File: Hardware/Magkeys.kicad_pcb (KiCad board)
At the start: 2 copper layers, 338 x 114.6 mm, 203 parts, among them SW1 SW_Push, SW10 SW_Push, SW100 SW_Push, SW101 SW_Push, SW11 SW_Push, SW12 SW_Push, SW13 SW_Push, SW14 SW_Push, SW15 SW_Push, SW16 SW_Push, SW17 SW_Push, SW18 SW_Push, SW19 SW_Push, SW2 SW_Push, SW20 SW_Push, SW21 SW_Push, SW22 SW_Push, SW23 SW_Push, SW24 SW_Push, SW25 SW_Push, SW26 SW_Push, SW27 SW_Push, SW28 SW_Push, SW29 SW_Push, SW3 SW_Push, SW30 SW_Push, SW31 SW_Push, SW32 SW_Push, SW33 SW_Push, SW34 SW_Push, SW35 SW_Push, SW36 SW_Push, SW37 SW_Push, SW38 SW_Push, SW39 SW_Push, SW4 SW_Push, SW40 SW_Push, SW41 SW_Push, SW42 SW_Push, SW43 SW_Push, SW44 SW_Push, SW45 SW_Push, SW46 SW_Push, SW47 SW_Push, SW48 SW_Push, SW49 SW_Push, SW5 SW_Push, SW50 SW_Push, SW51 SW_Push, SW52 SW_Push, SW53 SW_Push, SW54 SW_Push, SW55 SW_Push, SW56 SW_Push, SW57 SW_Push, SW58 SW_Push, SW59 SW_Push, SW6 SW_Push, SW60 SW_Push, SW61 SW_Push, SW62 SW_Push, SW63 SW_Push, SW64 SW_Push, SW65 SW_Push, SW66 SW_Push, SW67 SW_Push, SW68 SW_Push, SW69 SW_Push, SW7 SW_Push, SW70 SW_Push, SW71 SW_Push, SW72 SW_Push, SW73 SW_Push, SW74 SW_Push, SW75 SW_Push, SW76 SW_Push, SW77 SW_Push, SW78 SW_Push, SW79 SW_Push, SW8 SW_Push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

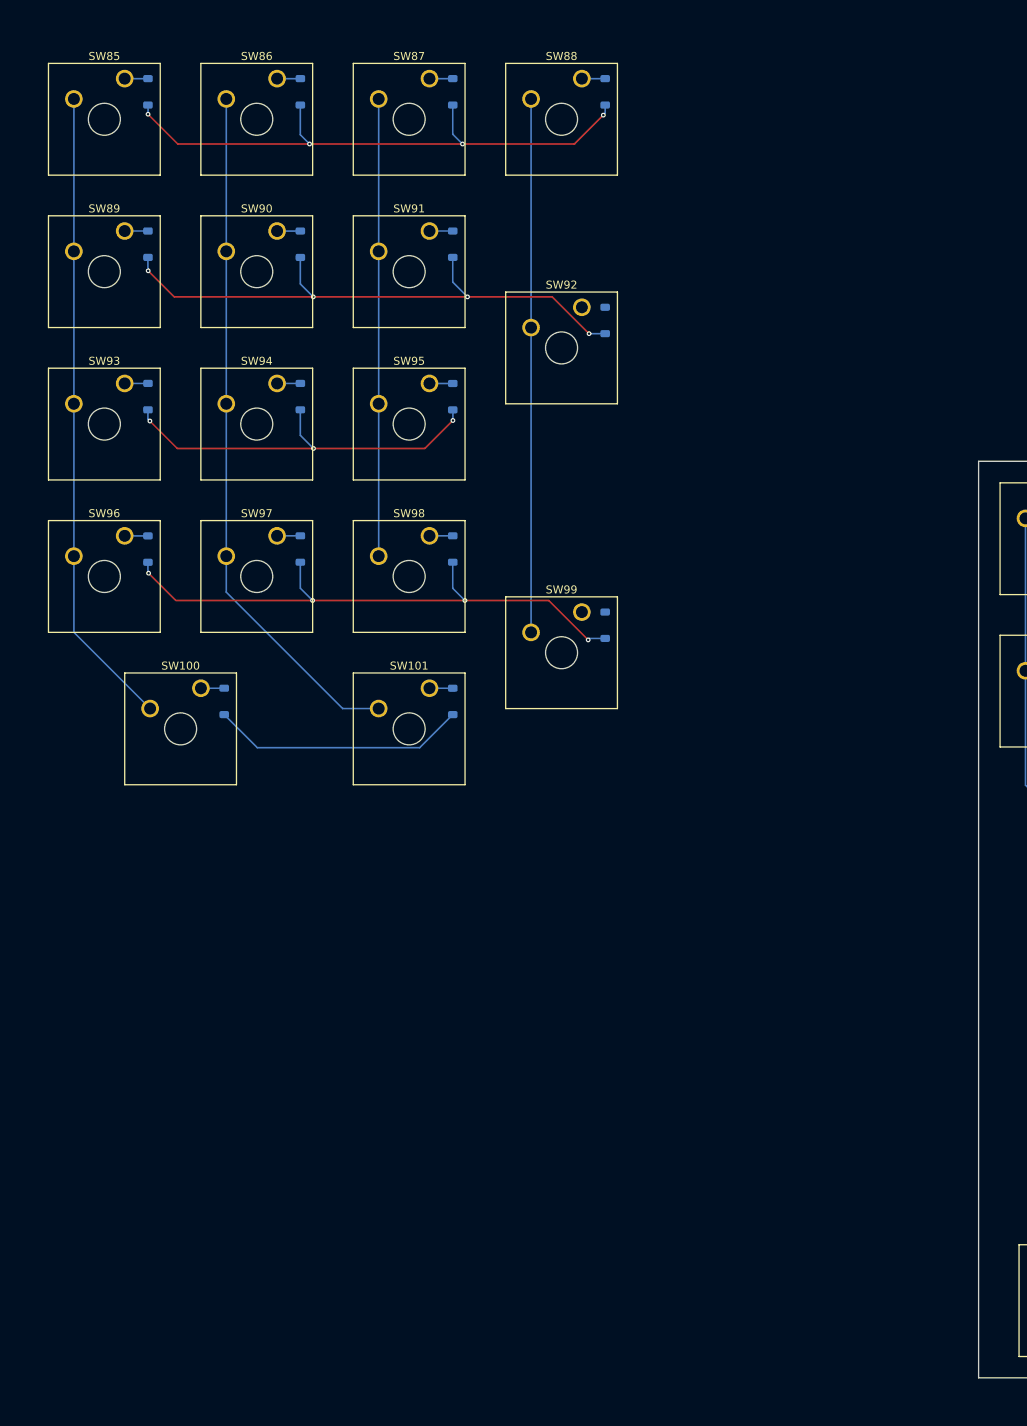
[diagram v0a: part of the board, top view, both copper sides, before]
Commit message: Completed PCB
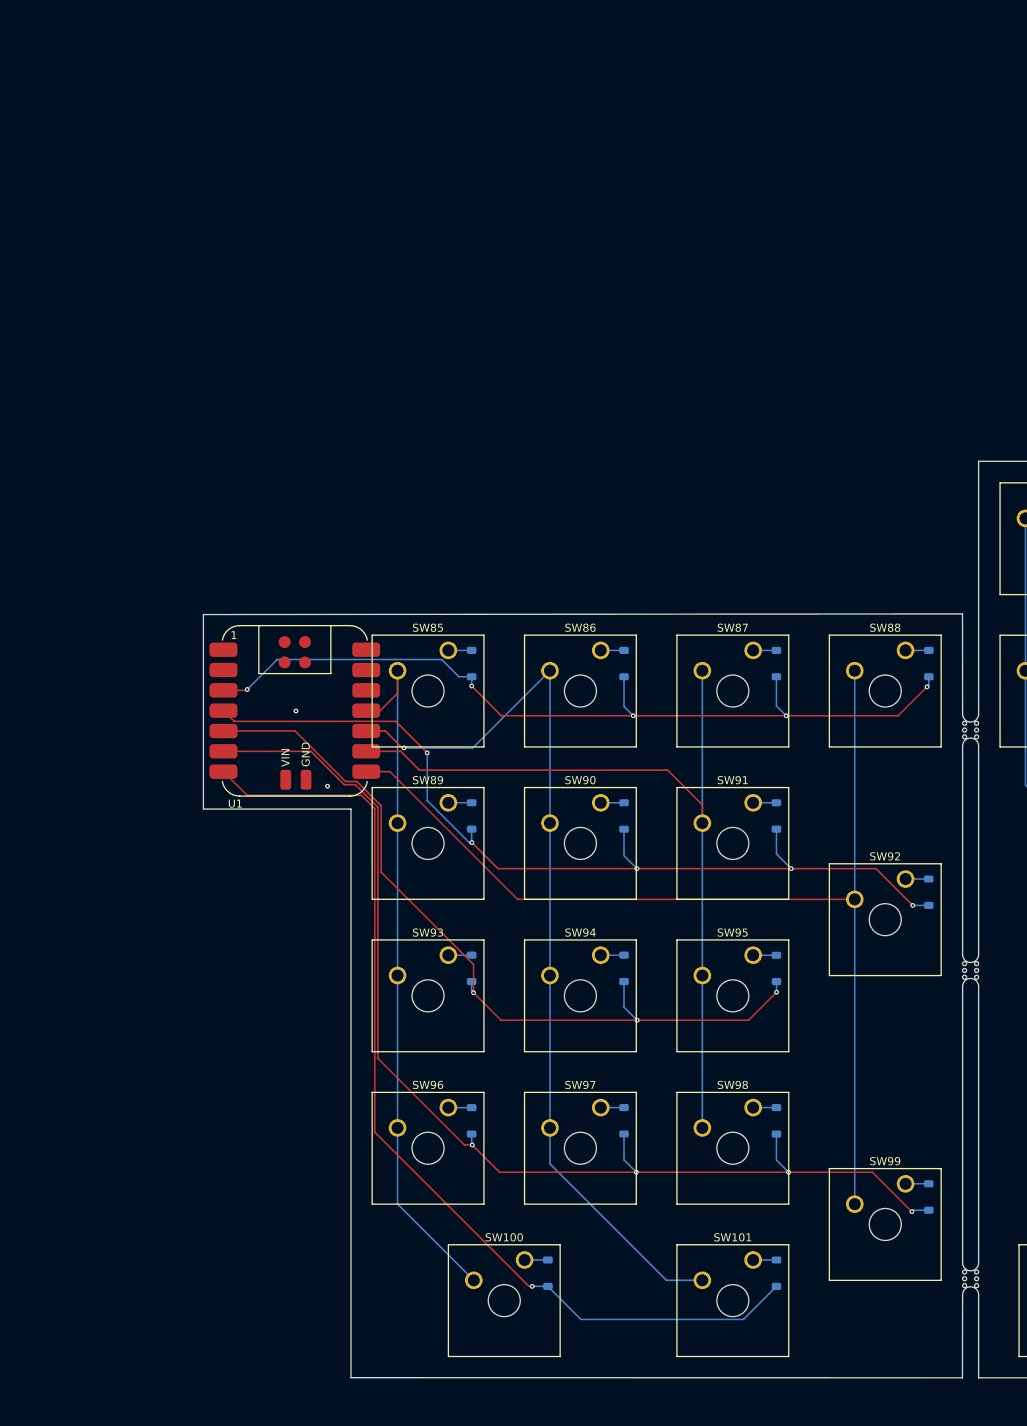
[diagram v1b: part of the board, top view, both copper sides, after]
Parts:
- added REF**: MouseBite-Slot_2.0x2.0mm_outset_D0.5mm_P0.85mm_3h, Panelization:MouseBite-Slot_2.0x2.0mm_outset_D0.5mm_P0.85mm_3h, F.Cu at (170.4, 215.1)
- added REF**: MouseBite-Slot_2.0x2.0mm_outset_D0.5mm_P0.85mm_3h, Panelization:MouseBite-Slot_2.0x2.0mm_outset_D0.5mm_P0.85mm_3h, F.Cu at (170.4, 253.7)
- added REF**: MouseBite-Slot_2.0x2.0mm_outset_D0.5mm_P0.85mm_3h, Panelization:MouseBite-Slot_2.0x2.0mm_outset_D0.5mm_P0.85mm_3h, F.Cu at (170.4, 185.1)
- added U1: Seeeduino Xiao rp2040, PCM_marbastlib-xp-promicroish:Xiao_rp2040_AC_Reflow, F.Cu at (84.9, 182.7)
- moved D88 82.1 mm to (164.2, 176.8)
- moved D90 82.1 mm to (126.1, 195.8)
- moved D92 82.1 mm to (164.2, 205.4)
- moved SW85 82.1 mm to (104.1, 175.1)
- moved SW88 82.1 mm to (161.3, 175.1)
- moved SW89 82.1 mm to (104.1, 194.2)
- moved SW90 82.1 mm to (123.2, 194.2)
- moved SW91 82.1 mm to (142.2, 194.2)
- moved SW92 82.1 mm to (161.3, 203.7)
- moved SW93 82.1 mm to (104.1, 213.2)
- moved SW96 82.1 mm to (104.1, 232.3)
- moved SW99 82.1 mm to (161.3, 241.8)
- moved D100 82.1 mm to (116.6, 253.0)
- moved D101 82.1 mm to (145.1, 253.0)
- moved D85 82.1 mm to (107.0, 176.8)
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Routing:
- net /NUM_ROW5: track 32.0 -> 122.9 mm, vias 0 -> 1
- net /NUM_ROW4: track 72.8 -> 142.7 mm
- net /NUM_COL4: track 66.7 -> 134.4 mm
- net /NUM_ROW3: track 49.1 -> 100.8 mm
- net /NUM_COL3: track 57.1 -> 105.1 mm
- net /NUM_ROW2: track 73.4 -> 114.7 mm, vias 4 -> 5
- net /NUM_ROW1: track 73.2 -> 106.7 mm, vias 4 -> 5
- net /NUM_COL2: track 86.7 -> 114.6 mm, vias 0 -> 1
- net /NUM_COL1: track 80.1 -> 87.8 mm
- net Net-(D99-A): track 0.00 -> 2.91 mm
- net Net-(D92-A): track 0.00 -> 2.91 mm
- net GND: vias 2 -> 4
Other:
- board size 338 x 114.6 mm -> 434.9 x 114.6 mm
